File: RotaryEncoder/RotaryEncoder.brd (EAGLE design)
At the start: 35.6 x 29.8 mm, 11 parts

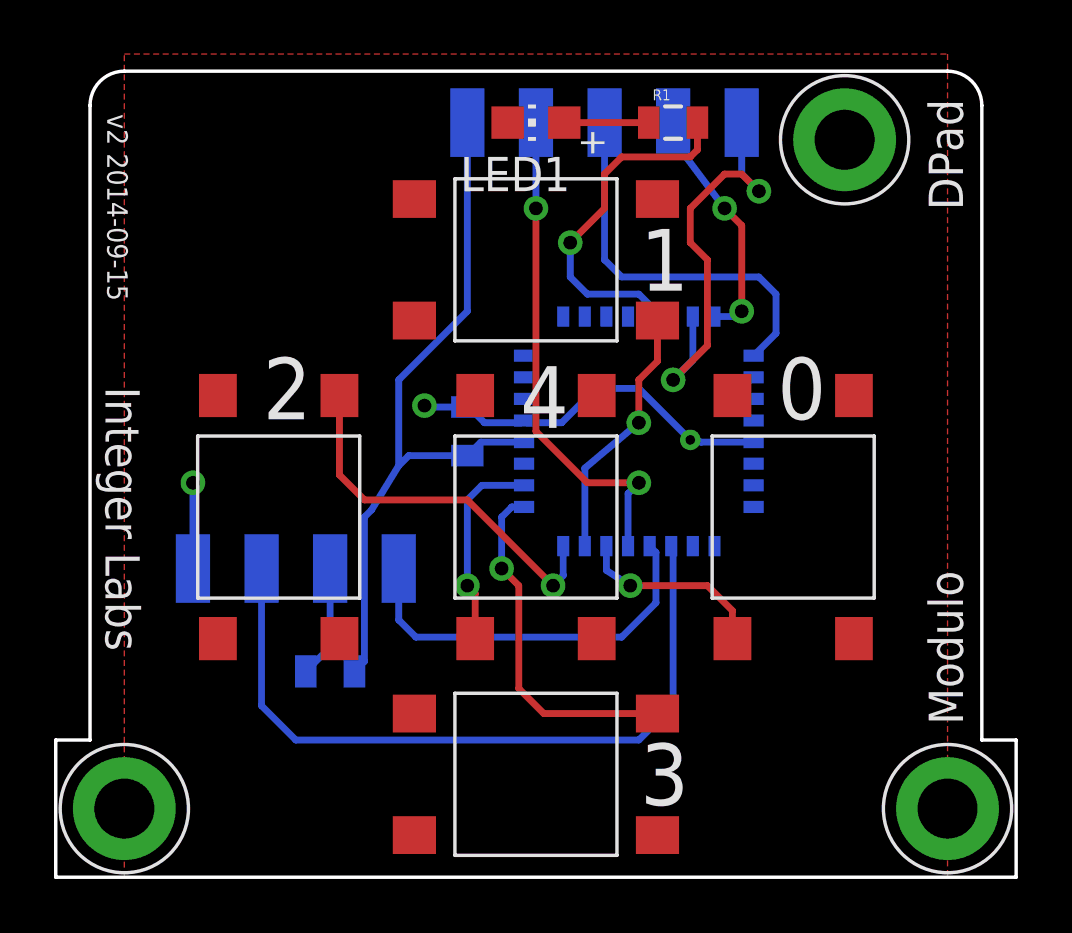
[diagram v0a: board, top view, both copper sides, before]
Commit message: Latest version of schematics and boards
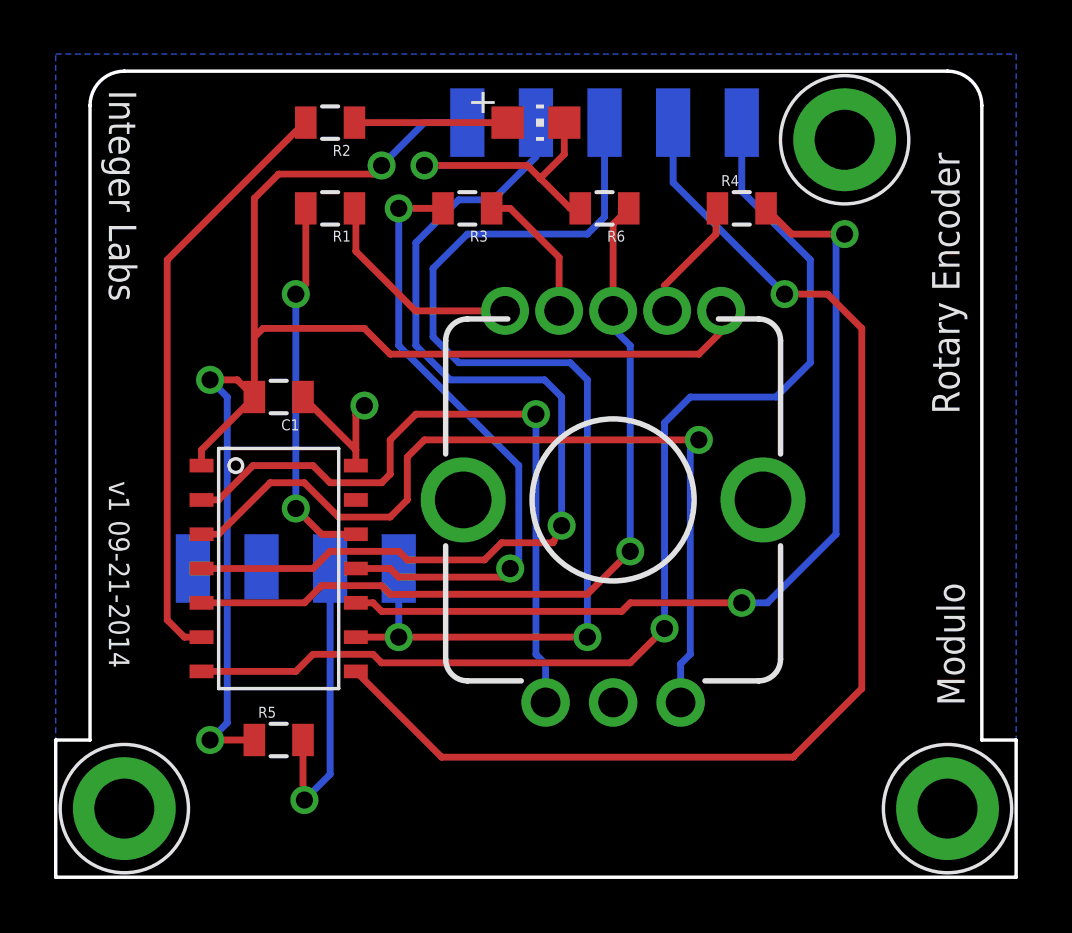
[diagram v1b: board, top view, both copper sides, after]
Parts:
- removed B1, B3, B4, B5, B7: TACT-SWITCH, IntegerLabs:MJTP1138
- removed U$5: ATTINY48/88-TQFP, IntegerLabs:TQFP-32
- added R3, R4: 68, SparkFun-Passives:0805
- added R5: 1, SparkFun-Passives:0805
- added R6: 2k, SparkFun-Passives:0805
- added SW1: (no value), SparkFun-Electromechanical:ENCODER_LED_3
- added U$1: TINY841, IntegerLabs:SOIC14
- R1: value 680 -> 120
- R2: value (none) -> 680; device SparkFun-Resistors:0805 -> SparkFun-Passives:0805
- moved R2 20.3 mm to (10.2, 27.9), flipped to the top, turned to 180 degrees
- moved R1 13.1 mm to (10.2, 24.8), turned to 180 degrees
- moved C1 7.10 mm to (8.26, 17.8), flipped to the top, turned to 180 degrees
- turned LED1 to 270 degrees
- renumbered U$2 to U$7
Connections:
- removed net AVCC: U$5.18
- removed net BUTTON0: B5.POS1, U$5.30
- removed net BUTTON1: B1.POS1, U$5.31
- removed net BUTTON2: B3.POS1, U$5.32
- removed net BUTTON3: B7.POS2, U$5.1
- removed net BUTTON4: B4.POS1, U$5.2
- removed net MOSI: U$5.15, U$7.PROG4
- removed net N$2: R2.2, U$7.BUS2
- removed net N$8: LED1.A, R1.1
- removed net SCK: U$5.17, U$7.PROG2
- removed net SCL: U$5.28, U$7.BUS3
- removed net THERM: U$5.25
- new net A: SW1.A, U$1.2
- new net B: SW1.B, U$1.3
- new net BLUE: R4.2, U$1.10
- new net GREEN: R3.2, U$1.11
- new net N$13: R5.2, U$7.BUS2
- new net N$4: R1.1, SW1.1
- new net N$5: R3.1, SW1.2
- new net N$6: R4.1, SW1.4
- new net N$7: LED1.A, R2.1
- new net RED: R1.2, U$1.12
- new net SCL/SCK: U$1.9, U$7.BUS3, U$7.PROG2
- new net SDA/MOSI: U$1.7, U$7.PROG4
- new net SW: R6.1, SW1.3, U$1.5
- net GND: now also R6.2, SW1.C, U$1.14; no longer B1.NEG2, B3.NEG2, B4.NEG2, B5.NEG2, B7.NEG2, U$5.21, U$5.5
- net LED: now also R2.2, U$1.6; no longer R1.2, U$5.13
- net MISO: now also U$1.8; no longer U$5.16
- net RESET: now also U$1.4; no longer U$5.29
- net SDA: no longer U$5.27
- net VCC: now also R5.1, SW1.5, U$1.1; no longer R2.1, U$5.4
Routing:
- net SDA/MOSI: track 0.00 -> 41.9 mm, vias 0 -> 1
- net SCL/SCK: track 0.00 -> 40.2 mm, vias 0 -> 2
- net MISO: track 8.97 -> 45.9 mm, vias 2 -> 1
- net BLUE: track 0.00 -> 33.6 mm, vias 0 -> 2
- net B: track 0.00 -> 31.8 mm, vias 0 -> 1
- net SW: track 0.00 -> 30.1 mm, vias 0 -> 1
- net VCC: track 26.9 -> 56.1 mm, vias 0 -> 3
- net SDA: track 27.3 -> 0.00 mm
- net A: track 0.00 -> 25.8 mm, vias 0 -> 1
- net GREEN: track 0.00 -> 22.9 mm, vias 0 -> 2
- net RESET: track 18.5 -> 36.2 mm, vias 2 -> 1
- net MOSI: track 15.9 -> 0.00 mm, vias 2 -> 0
- net SCK: track 14.6 -> 0.00 mm
- net SCL: track 14.4 -> 0.00 mm
- net BUTTON2: track 14.2 -> 0.00 mm, vias 1 -> 0
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- added copper zone on layer 16, net GND
- removed copper zone on layer 1, net GND
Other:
- board text added: "Rotary Encoder"
- board text added: "v1 09-21-2014"
- board text removed: "0"
- board text removed: "1"
- board text removed: "2"
- board text removed: "3"
- board text removed: "4"
- board text removed: "DPad"
- board text removed: "v2 2014-09-15"
